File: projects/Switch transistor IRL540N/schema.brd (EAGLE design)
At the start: 160 x 100 mm, 6 parts, among them Q1 IRF3704L-V

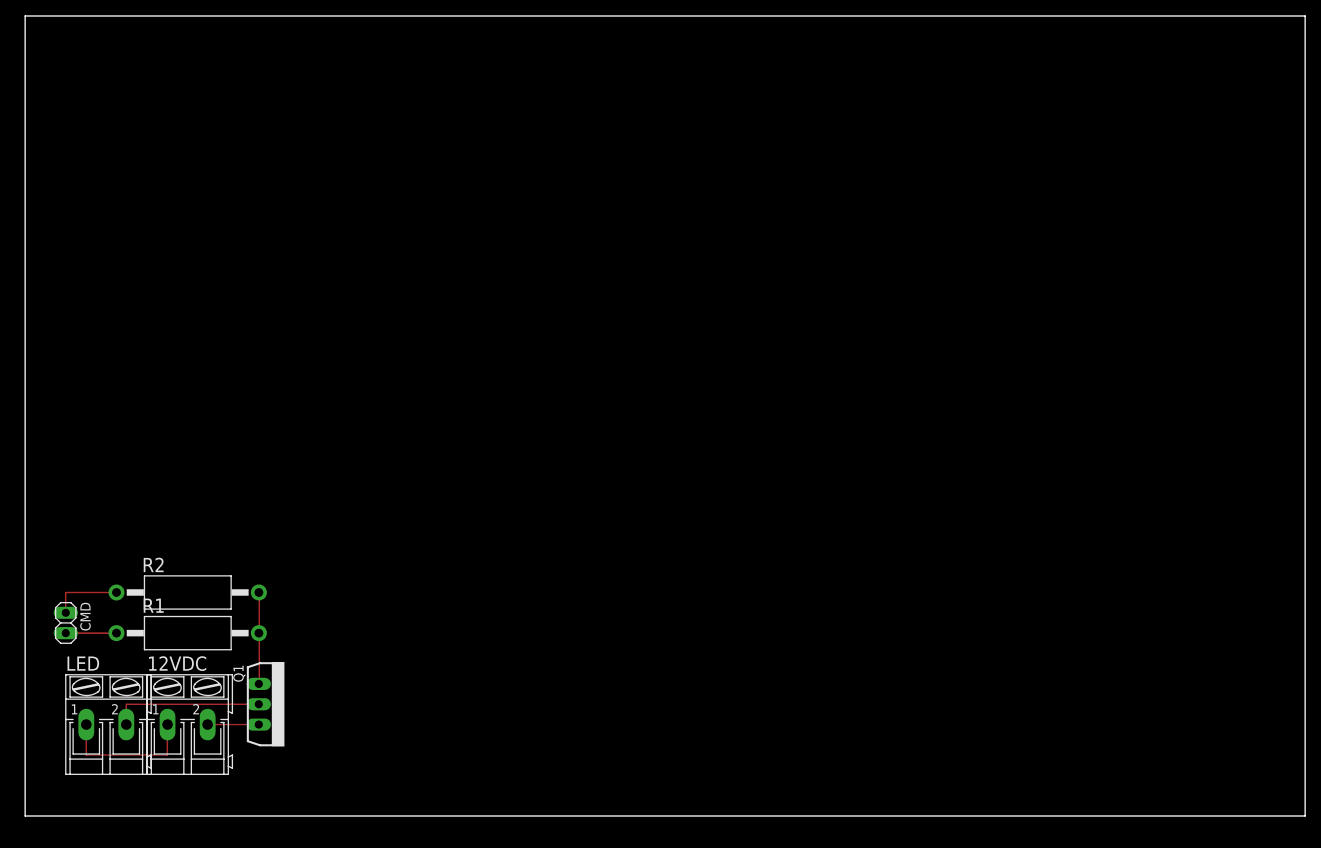
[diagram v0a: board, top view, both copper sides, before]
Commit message: rinominato progetto switch.
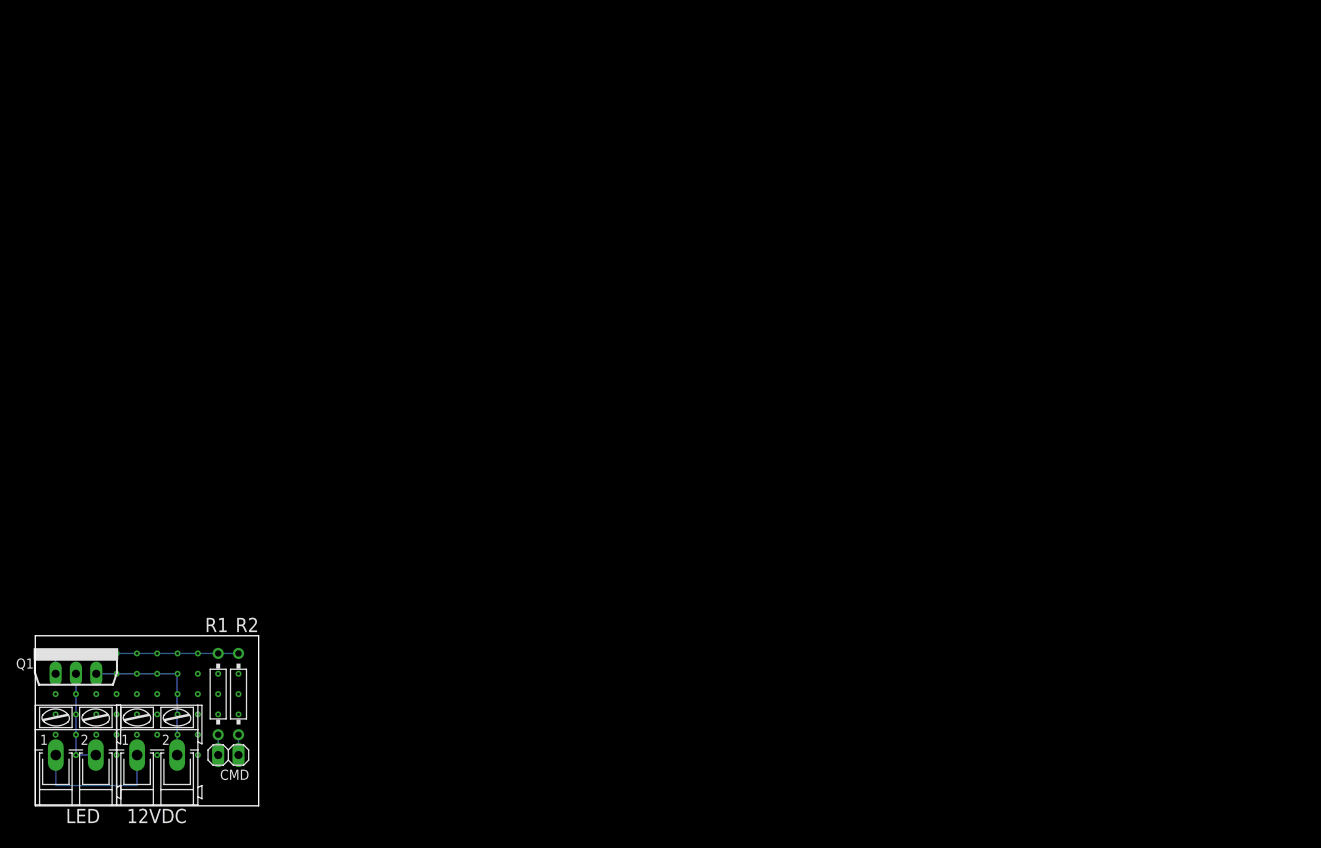
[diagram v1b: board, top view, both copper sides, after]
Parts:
- Q1: value IRF3704L-V -> IRL540N
- R1, R2: device resistor-power:AC01 -> resistor-power:RS1/4
- moved CMD 26.2 mm to (25.4, 7.62), turned to 180 degrees
- moved Q1 23.2 mm to (6.35, 17.8), turned to 0 degrees
- moved R2 14.2 mm to (26.7, 15.2), turned to 90 degrees
- moved R1 8.52 mm to (24.1, 15.2), turned to 90 degrees
- moved LED 5.39 mm to (6.35, 7.62)
- moved 12VDC 5.39 mm to (16.5, 7.62)
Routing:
- net N$2: track 11.5 -> 25.4 mm, vias 0 -> 8
- net N$6: track 6.40 -> 20.3 mm, vias 0 -> 3
- net N$3: track 9.14 -> 2.54 mm
- net N$5: track 19.2 -> 12.6 mm, vias 0 -> 4
- net N$1: track 6.34 -> 2.54 mm
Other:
- board size 160 x 100 mm -> 27.9 x 21.3 mm
